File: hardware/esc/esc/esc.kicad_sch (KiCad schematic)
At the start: 9 parts, among them IC1 XMC1100T016F0016ABXUMA1, IC2 STDRIVE101TR, Q1 BSC030P03NS3G, Q2 BSC030P03NS3G, Q3 BSC030P03NS3G, Q4 BSC030P03NS3G, Q5 BSC030P03NS3G, Q6 BSC030P03NS3G, U1 AP62300Z6

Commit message: hardware edits mainly
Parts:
- removed IC1: XMC1100T016F0016ABXUMA1, SOP65P640X120-16N, symbol XMC1100T016F0016ABXUMA1:XMC1100T016F0016ABXUMA1
- removed IC2: STDRIVE101TR, QFN50P400X400X100-25N-D, symbol STDRIVE101TR:STDRIVE101TR
- removed Q1, Q2, Q3, Q4, Q5, Q6: BSC030P03NS3G, BSC0902NSATMA1, symbol BSC030N03LSGATMA1:BSC030P03NS3G
- removed U1: AP62300Z6, Package_TO_SOT_SMD:SOT-563, symbol Regulator_Switching:AP62300Z6
- added C1, C10, C11, C16, C17, C18, C23, C24, C25, C3, C30, C31, C32, C39, C40, C41, C43, C44, C45, C46, C48, C5, C50, C51, C54, C55, C57, C58, C60, C61, C63, C64, C66, C67, C71, C72, C73, C74, C75, C76, C84, C85, C88, C9, C91: 4.7uF, Capacitor_SMD:CP_Elec_6.3x7.7, symbol Device:C_Small
- added C12, C13, C14, C19, C2, C20, C21, C26, C27, C28, C33, C34, C35, C36, C37, C38, C4, C52, C53, C56, C59, C6, C62, C65, C83, C86, C89, C92: 220nF, Capacitor_SMD:C_0402_1005Metric, symbol Device:C_Small
- added C15, C22, C29, C42, C7, C8: 1nF, Capacitor_SMD:C_0603_1608Metric, symbol Device:C_Small
- added C47, C49: 18pF, Capacitor_SMD:C_0402_1005Metric, symbol Device:C_Small
- added C68: 1uF, Capacitor_SMD:C_0603_1608Metric, symbol Device:C_Small
- added C69, C70, C77, C78, C79, C80, C81, C82, C87, C90, C93: 0.1uF, Capacitor_SMD:C_0603_1608Metric, symbol Device:C_Small
- added D1, D10, D11, D12, D13, D14, D15, D16, D17, D18, D19, D2, D3, D4, D5, D6, D7, D8, D9: D_Small, Diode_SMD:D_SMA, symbol Device:D_Small
- added IC1, IC2, IC3, IC4, IC5, IC6: IR2136SPBF, SOIC127P1032X265-28N, symbol IR2136SPBF:IR2136SPBF
- added IC7: TLA2528IRTER, Package_DFN_QFN:WQFN-16-1EP_3x3mm_P0.5mm_EP1.68x1.68mm_ThermalVias, symbol TLA2528IRTER:TLA2528IRTER
- added IC8: MP9486AGN-Z, Package_SO:SOIC-8-1EP_3.9x4.9mm_P1.27mm_EP2.62x3.51mm_ThermalVias, symbol MP9486AGN-Z:MP9486AGN-Z
- added J1: USB-C, Connector_PinHeader_2.54mm:PinHeader_1x04_P2.54mm_Vertical, symbol Connector:Conn_01x04_Pin
- added J10: GPIO, Connector_PinHeader_2.54mm:PinHeader_1x04_P2.54mm_Vertical, symbol Connector:Conn_01x04_Pin
- added J11: Conn_01x08_Pin, Connector_PinHeader_1.27mm:PinHeader_1x08_P1.27mm_Vertical, symbol Connector:Conn_01x08_Pin
- added J2: DEBUG, Connector_PinHeader_2.54mm:PinHeader_1x04_P2.54mm_Vertical, symbol Connector:Conn_01x04_Pin
- added J3: TEMP-GPIO, Connector_PinHeader_1.27mm:PinHeader_1x08_P1.27mm_Vertical, symbol Connector:Conn_01x08_Pin
- added L1: 3.3uH, Inductor_SMD:L_0805_2012Metric_Pad1.05x1.20mm_HandSolder, symbol Device:L_Small
- added L2: 33uH, Inductor_SMD:L_0805_2012Metric, symbol Device:L_Small
- added Q1, Q10, Q11, Q12, Q13, Q14, Q15, Q16, Q17, Q18, Q19, Q2, Q20, Q21, Q22, Q23, Q24, Q25, Q26, Q27, Q28, Q29, Q3, Q30, Q31, Q32, Q33, Q34, Q35, Q36, Q4, Q5, Q6, Q7, Q8, Q9: NMOS, Package_SO:PowerPAK_SO-8L_Single, symbol Simulation_SPICE:NMOS
- added R1, R2, R22, R23, R24, R25, R26, R27, R3, R34, R35, R36, R37, R38, R39, R4, R46, R47, R48, R49, R5, R50, R51, R58, R59, R6, R60, R61, R62, R63, R79, R80, R81, R82, R83, R84: 10, Resistor_SMD:R_1206_3216Metric, symbol Device:R_Small
- added R10, R11, R12, R13, R14, R15, R19, R20, R21, R31, R32, R33, R43, R44, R45, R55, R56, R57, R64, R65, R66, R67, R68, R69, R70, R71, R72, R73, R74, R75, R76, R77, R78: SHUNT, Fuse:Fuse_1206_3216Metric_Pad1.42x1.75mm_HandSolder, symbol Device:R_Small
- added R16, R17, R18, R28, R29, R30, R40, R41, R42, R52, R53, R54, R7, R8, R88, R89, R9, R90: 4.7, Resistor_SMD:R_0805_2012Metric, symbol Device:R_Small
- added R91, R92: 27, Resistor_SMD:R_0402_1005Metric, symbol Device:R_Small
- added R93, R94: 1k, Resistor_SMD:R_0201_0603Metric, symbol Device:R_Small
- added R95: 33, Resistor_SMD:R_1206_3216Metric, symbol Device:R_Small
- added R96: 240k, Resistor_SMD:R_0402_1005Metric, symbol Device:R_Small
- added R97, R98: 10k, Resistor_SMD:R_0402_1005Metric, symbol Device:R_Small
- added SW1, SW2: SW_Push, Connector_PinHeader_2.54mm:PinHeader_1x02_P2.54mm_Vertical, symbol Switch:SW_Push
- added TP1, TP10, TP11, TP12, TP13, TP14, TP15, TP16, TP17, TP18, TP2, TP3, TP4, TP5, TP6, TP7, TP8, TP9: TestPoint_Small, TestPoint:TestPoint_Pad_4.0x4.0mm, symbol Connector:TestPoint_Small
- added TP19, TP20, TP21, TP22: TestPoint, TestPoint:TestPoint_Pad_4.0x4.0mm, symbol Connector:TestPoint
- added U1: RP2354B, Package_DFN_QFN:QFN-80-1EP_10x10mm_P0.4mm_EP3.4x3.4mm, symbol MCU_RaspberryPi:RP2354B
- added U10, U11, U12, U2, U3, U4, U5, U6, U7, U8, U9: INA240A2PW, Package_SO:TSSOP-8_4.4x3mm_P0.65mm, symbol Amplifier_Current:INA240A2PW
- added U14, U15: TMP110D, Package_SON:Texas_X2SON-5_0.8x0.8mm_P0.48mm, symbol Sensor_Temperature:TMP110D
- added U16: AZ1117CH2-3.3, Package_TO_SOT_SMD:SOT-223-3_TabPin2, symbol Regulator_Linear:AZ1117CH2-3.3
- added Y1: 12MHz, Crystal:Crystal_SMD_ECS_CSM3X-2Pin_7.6x4.1mm, symbol Device:Crystal
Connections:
- new net: C49.2, U1.30 (XIN), Y1.2
- new net: C16.1, C19.1, IC3.22 (VS2), Q15.1 (S), Q15.2 (S), Q15.3 (S), Q16.5 (D), TP8.1
- new net: C16.2, C19.2, IC3.24 (VB2), R29.1
- new net: Q10.1 (S), Q10.2 (S), Q10.3 (S), Q12.1 (S), Q12.2 (S), Q12.3 (S), Q8.1 (S), Q8.2 (S), Q8.3 (S), R19.2, R20.2, R21.2, U4.2 (+)
- new net: J1.2 (Pin_2), R91.2
- new net: J1.3 (Pin_3), R92.1
- new net: C11.2, C14.2, IC2.20 (VB3), R18.1
- new net: D5.1 (K), R18.2
- new net: Q4.1 (S), Q4.2 (S), Q4.3 (S), Q5.1 (S), Q5.2 (S), Q5.3 (S), Q6.1 (S), Q6.2 (S), Q6.3 (S), R10.2, R11.2, R12.2, U2.2 (+)
- new net: Q4.4 (G), R4.2
- new net: C5.2, C6.1, IC1.18 (VS3), Q1.1 (S), Q1.2 (S), Q1.3 (S), Q4.5 (D), TP6.1
- new net: C30.1, C33.1, IC5.22 (VS2), Q27.1 (S), Q27.2 (S), Q27.3 (S), Q28.5 (D), TP18.1
- new net: C30.2, C33.2, IC5.24 (VB2), R53.1
- new net: C32.2, C35.2, IC5.20 (VB3), R54.1
- new net: D14.1 (K), R54.2
- new net: C17.1, C20.1, IC3.28 (VB1), R28.1
- new net: C17.2, C20.2, IC3.26 (VS1), Q17.1 (S), Q17.2 (S), Q17.3 (S), Q18.5 (D), TP7.1
- new net: Q35.1 (S), Q35.2 (S), Q35.3 (S), R76.2, R77.2, R78.2, U12.2 (+)
- new net: Q35.4 (G), R84.2
- new net: C36.1, C39.1, IC6.18 (VS3), Q35.5 (D), Q36.1 (S), Q36.2 (S), Q36.3 (S), TP15.1
- new net: IC1.23 (HO2), R2.1
- new net: Q2.4 (G), R2.2
- new net: IC2.15 (LO2), R24.1
- new net: Q10.4 (G), R24.2
- new net: Q28.1 (S), Q28.2 (S), Q28.3 (S), R67.2, R68.2, R69.2, U8.2 (+)
- new net: Q28.4 (G), R60.2
- new net: Q20.1 (S), Q20.2 (S), Q20.3 (S), Q22.1 (S), Q22.2 (S), Q22.3 (S), Q24.1 (S), Q24.2 (S), Q24.3 (S), R43.2, R44.2, R45.2, U6.2 (+)
- new net: C47.2, U1.31 (XOUT), Y1.1
- new net: C29.1, IC5.11 (RCIN)
- new net: R93.2, SW1.1, SW2.1, U1.35 (RUN)
- new net: R94.1, SW2.2
- new net: Q36.4 (G), R83.2
- new net: IC2.23 (HO2), R26.1
- new net: Q9.4 (G), R26.2
- new net: D15.1 (K), R53.2
- new net: C22.1, IC4.11 (RCIN)
- new net: C23.1, C26.1, IC4.22 (VS2), Q21.1 (S), Q21.2 (S), Q21.3 (S), Q22.5 (D), TP11.1
- new net: C23.2, C26.2, IC4.24 (VB2), R41.1
- new net: Q17.4 (G), R39.2
- new net: C31.1, C34.1, IC5.28 (VB1), R52.1
- new net: C31.2, C34.2, IC5.26 (VS1), Q29.1 (S), Q29.2 (S), Q29.3 (S), Q30.5 (D), TP17.1
- new net: C10.2, C13.2, IC2.26 (VS1), Q11.1 (S), Q11.2 (S), Q11.3 (S), Q12.5 (D), TP1.1
- new net: Q31.1 (S), Q31.2 (S), Q31.3 (S), R13.2, R14.2, R15.2, U10.2 (+)
- new net: C25.1, C28.1, IC4.18 (VS3), Q19.1 (S), Q19.2 (S), Q19.3 (S), Q20.5 (D), TP12.1
- new net: Q19.4 (G), R47.2
- new net: IC3.27 (HO1), R39.1
- new net: C12.2, C9.1, IC2.24 (VB2), R17.1
- new net: D6.1 (K), R17.2
- new net: IC5.19 (HO3), R59.1
- new net: Q25.4 (G), R59.2
- new net: Q14.1 (S), Q14.2 (S), Q14.3 (S), Q16.1 (S), Q16.2 (S), Q16.3 (S), Q18.1 (S), Q18.2 (S), Q18.3 (S), R31.2, R32.2, R33.2, U5.2 (+)
- new net: Q18.4 (G), R37.2
- new net: IC7.13 (SCL), U1.12 (GPIO13), U14.2 (SCL), U15.2 (SCL)
- new net: U1.13 (GPIO14), U14.3 (ADD0)
- new net: IC7.14 (SDA), U1.11 (GPIO12), U14.4 (SDA), U15.4 (SDA)
- new net: Q5.4 (G), R5.2
- new net: C3.2, C4.1, IC1.22 (VS2), Q2.1 (S), Q2.2 (S), Q2.3 (S), Q5.5 (D), TP5.1
- new net: C24.2, C27.2, IC4.26 (VS1), Q23.1 (S), Q23.2 (S), Q23.3 (S), Q24.5 (D), TP10.1
- new net: C25.2, C28.2, IC4.20 (VB3), R42.1
- new net: D11.1 (K), R42.2
- new net: C18.1, C21.1, IC3.18 (VS3), Q13.1 (S), Q13.2 (S), Q13.3 (S), Q14.5 (D), TP9.1
- new net: C18.2, C21.2, IC3.20 (VB3), R30.1
- new net: C36.2, C39.2, IC6.20 (VB3), R88.1
- new net: C37.2, C40.2, IC6.26 (VS1), Q31.5 (D), Q32.1 (S), Q32.2 (S), Q32.3 (S), TP13.1
- new net: D9.1 (K), R29.2
- new net: D3.1 (K), R9.2
- new net: Q8.4 (G), R22.2
- new net: C11.1, C14.1, IC2.18 (VS3), Q7.1 (S), Q7.2 (S), Q7.3 (S), Q8.5 (D), TP3.1
- new net: Q33.1 (S), Q33.2 (S), Q33.3 (S), R73.2, R74.2, R75.2, U11.2 (+)
- new net: R55.2, R56.2, R57.2, R64.1, R65.1, R66.1, R67.1, R68.1, R69.1, R70.1, R71.1, R72.1, U7.2 (+)
- new net: Q30.1 (S), Q30.2 (S), Q30.3 (S), R64.2, R65.2, R66.2, U3.2 (+)
- new net: Q6.4 (G), R6.2
- new net: C1.2, C2.2, IC1.26 (VS1), Q3.1 (S), Q3.2 (S), Q3.3 (S), Q6.5 (D), TP4.1
- new net: C1.1, C2.1, IC1.28 (VB1), R8.1
- new net: R93.1, U1.75 (~{QSPI_SS})
- new net: Q29.4 (G), R63.2
- new net: D18.1 (K), R90.2
- new net: C38.1, C41.1, IC6.22 (VS2), Q33.5 (D), Q34.1 (S), Q34.2 (S), Q34.3 (S), TP14.1
- new net: Q34.4 (G), R80.2
- new net: IC8.6 (DIM), IC8.7 (EN), R98.1
- new net: Q26.1 (S), Q26.2 (S), Q26.3 (S), R70.2, R71.2, R72.2, U9.2 (+)
- new net: IC4.23 (HO2), R50.1
- new net: Q21.4 (G), R50.2
- new net: C38.2, C41.2, IC6.24 (VB2), R89.1
- new net: C42.1, IC6.11 (RCIN)
- new net: Q22.4 (G), R48.2
- new net: IC6.15 (LO2), R82.1
- new net: Q33.4 (G), R82.2
- new net: D1.1 (K), R8.2
- new net: D12.1 (K), R41.2
- new net: C44.1, R95.1, U1.61 (VREG_AVDD)
- new net: IC5.14 (LO3), R61.1
- new net: Q30.4 (G), R61.2
- new net: IC4.16 (LO1), R46.1
- new net: Q20.4 (G), R46.2
- new net: Q26.4 (G), R58.2
- new net: C32.1, C35.1, IC5.18 (VS3), Q25.1 (S), Q25.2 (S), Q25.3 (S), Q26.5 (D), TP16.1
- new net: C77.1, U16.2 (GND)
- new net: IC4.15 (LO2), R48.1
- new net: IC7.15 (AIN0/GPIO0), J3.1 (Pin_1)
- new net: IC7.16 (AIN1/GPIO1), J3.2 (Pin_2)
- new net: IC7.1 (AIN2/GPIO2), J3.3 (Pin_3)
- new net: IC7.2 (AIN3/GPIO3), J3.4 (Pin_4)
- new net: IC7.3 (AIN4/GPIO4), J3.5 (Pin_5)
- new net: IC7.4 (AIN5/GPIO5), J3.6 (Pin_6)
- new net: IC7.5 (AIN6/GPIO6), J3.7 (Pin_7)
- new net: IC7.6 (AIN7/GPIO7), J3.8 (Pin_8)
- new net: IC2.14 (LO3), R25.1
- new net: Q12.4 (G), R25.2
- new net: IC1.9 (ITRIP), U1.4 (GPIO7), U2.8
- new net: U1.54 (GPIO43/ADC3), U10.8
- new net: Q31.4 (G), R81.2
- new net: D4.1 (K), R16.2
- new net: C10.1, C13.1, IC2.28 (VB1), R16.1
- new net: IC3.10 (EN), U1.44 (GPIO35)
- new net: C15.1, IC3.11 (RCIN)
- new net: IC3.14 (LO3), R37.1
- new net: IC3.15 (LO2), R36.1
- new net: IC3.16 (LO1), R34.1
- new net: IC3.19 (HO3), R35.1
- new net: IC3.2 (~{HIN1}), IC4.2 (~{HIN1}), IC5.2 (~{HIN1}), U1.38 (GPIO30)
- new net: IC3.23 (HO2), R38.1
- new net: IC3.3 (~{HIN2}), IC4.3 (~{HIN2}), IC5.3 (~{HIN2}), U1.40 (GPIO32)
- new net: IC3.4 (~{HIN3}), IC4.4 (~{HIN3}), IC5.4 (~{HIN3}), U1.43 (GPIO34)
- new net: IC3.5 (~{LIN1}), IC4.5 (~{LIN1}), IC5.5 (~{LIN1}), U1.45 (GPIO36)
- new net: IC3.6 (~{LIN2}), IC4.6 (~{LIN2}), IC5.6 (~{LIN2}), U1.47 (GPIO38)
- new net: IC3.7 (~{LIN3}), IC4.7 (~{LIN3}), IC5.7 (~{LIN3}), U1.48 (GPIO39)
- new net: IC3.8 (~{FAULT}), U1.46 (GPIO37)
- new net: IC3.9 (ITRIP), U1.26 (GPIO25), U5.8
- new net: IC1.14 (LO3), R6.1
- new net: C70.2, IC8.1 (FB), R96.1, R97.2
- new net: Q1.4 (G), R3.2
- new net: C24.1, C27.1, IC4.28 (VB1), R40.1
- new net: Q14.4 (G), R34.2
- new net: C37.1, C40.1, IC6.28 (VB1), R90.1
- new net: D13.1 (K), R52.2
- new net: Q32.4 (G), R79.2
- new net: C68.1, IC7.8 (DECAP)
- new net: IC6.23 (HO2), R80.1
- new net: Q3.4 (G), R1.2
- new net: IC2.10 (EN), U1.9 (GPIO11)
- new net: C8.1, IC2.11 (RCIN)
- new net: IC2.16 (LO1), R22.1
- new net: IC2.19 (HO3), R23.1
- new net: IC1.2 (~{HIN1}), IC2.2 (~{HIN1}), IC6.2 (~{HIN1}), U1.77 (GPIO0)
- new net: C12.1, C9.2, IC2.22 (VS2), Q10.5 (D), Q9.1 (S), Q9.2 (S), Q9.3 (S), TP2.1
- new net: IC2.27 (HO1), R27.1
- new net: IC1.3 (~{HIN2}), IC2.3 (~{HIN2}), IC6.3 (~{HIN2}), U1.79 (GPIO2)
- new net: IC1.4 (~{HIN3}), IC2.4 (~{HIN3}), IC6.4 (~{HIN3}), U1.1 (GPIO4)
- new net: IC1.5 (~{LIN1}), IC2.5 (~{LIN1}), IC6.5 (~{LIN1}), U1.3 (GPIO6)
- new net: IC1.6 (~{LIN2}), IC2.6 (~{LIN2}), IC6.6 (~{LIN2}), U1.6 (GPIO8)
- new net: IC1.7 (~{LIN3}), IC2.7 (~{LIN3}), IC6.7 (~{LIN3}), U1.8 (GPIO10)
- new net: IC2.8 (~{FAULT}), U1.7 (GPIO9)
- new net: IC2.9 (ITRIP), U1.58 (GPIO47/ADC7), U4.8
- new net: D16.1 (K), R89.2
- new net: L1.2, U1.63 (VREG_LX)
- new net: C5.1, C6.2, IC1.20 (VB3), R9.1
- new net: IC4.14 (LO3), R49.1
- new net: Q24.4 (G), R49.2
- new net: IC1.15 (LO2), R5.1
- new net: D17.1 (K), R88.2
- new net: U1.14 (GPIO15), U15.3 (ADD0)
- new net: IC7.11 (ADDR), U1.2 (GPIO5)
- new net: C69.1, D19.1 (K), IC8.5 (SW), L2.2
- new net: C69.2, IC8.4 (BST)
- new net: C3.1, C4.2, IC1.24 (VB2), R7.1
- new net: IC1.19 (HO3), R3.1
- new net: D2.1 (K), R7.2
- new net: IC6.16 (LO1), R84.1
- new net: D10.1 (K), R40.2
- new net: U1.56 (GPIO45/ADC5), U12.8
- new net: Q27.4 (G), R62.2
- new net: IC5.9 (ITRIP), U7.8
- new net: IC6.27 (HO1), R79.1
- new net: IC1.16 (LO1), R4.1
- new net: IC4.27 (HO1), R51.1
- new net: Q23.4 (G), R51.2
- new net: Q16.4 (G), R36.2
- new net: U1.53 (GPIO42/ADC2), U9.8
- new net: Q13.4 (G), R35.2
- new net: IC1.27 (HO1), R1.1
- new net: Q11.4 (G), R27.2
- new net: IC5.27 (HO1), R63.1
- new net: R92.2, U1.67 (USB_DP)
- new net: J11.3 (Pin_3), U1.25 (GPIO24)
- new net: J11.4 (Pin_4), U1.23 (GPIO23)
- new net: J11.5 (Pin_5), U1.22 (GPIO22)
- new net: J11.6 (Pin_6), U1.21 (GPIO21)
- new net: IC4.9 (ITRIP), U1.57 (GPIO46/ADC6), U6.8
- new net: J2.3 (Pin_3), U1.33 (SWCLK)
- new net: J2.4 (Pin_4), U1.34 (SWDIO)
- new net: J10.1 (Pin_1), U1.19 (GPIO19)
- new net: J10.2 (Pin_2), U1.18 (GPIO18)
- new net: J10.3 (Pin_3), U1.17 (GPIO17)
- new net: J10.4 (Pin_4), U1.16 (GPIO16)
- new net: IC4.19 (HO3), R47.1
- new net: IC1.10 (EN), U1.80 (GPIO3)
- new net: C7.1, IC1.11 (RCIN)
- new net: IC1.8 (~{FAULT}), U1.78 (GPIO1)
- new net: IC5.10 (EN), U1.36 (GPIO28)
- new net: IC5.15 (LO2), R60.1
- new net: IC5.16 (LO1), R58.1
- new net: IC5.23 (HO2), R62.1
- new net: IC5.8 (~{FAULT}), U1.37 (GPIO29)
- new net: D7.1 (K), R28.2
- new net: D8.1 (K), R30.2
- new net: Q15.4 (G), R38.2
- new net: R91.1, U1.66 (USB_DM)
- new net: IC4.10 (EN), U1.39 (GPIO31)
- new net: IC4.8 (~{FAULT}), U1.42 (GPIO33)
- new net: IC6.8 (~{FAULT}), U1.27 (GPIO26)
- new net: IC6.10 (EN), U1.28 (GPIO27)
- new net: U1.49 (GPIO40/ADC0), U3.8
- new net: U1.52 (GPIO41/ADC1), U8.8
- new net: U1.55 (GPIO44/ADC4), U11.8
- new net: Q7.4 (G), R23.2
- new net: IC6.14 (LO3), R81.1
- new net: IC6.19 (HO3), R83.1
- new net +1V1: C43.2, C46.2, J2.1 (Pin_1), L1.1, U1.10 (DVDD), U1.32 (DVDD), U1.51 (DVDD), U1.65 (VREG_FB)
- new net +3V3: C45.1, C48.2, C50.1, C51.1, C52.1, C53.1, C54.1, C55.1, C56.1, C57.1, C58.1, C59.1, C60.1, C61.1, C62.1, C63.1, C64.1, C65.1, C66.1, C67.1, C77.2, C78.2, C79.2, C80.2, C81.2, D1.2 (A), D10.2 (A), D11.2 (A), D12.2 (A), D13.2 (A), D14.2 (A), D15.2 (A), D16.2 (A), D17.2 (A), D18.2 (A), D2.2 (A), D3.2 (A), D4.2 (A), D5.2 (A), D6.2 (A), D7.2 (A), D8.2 (A), D9.2 (A), IC1.1 (VCC), IC2.1 (VCC), IC3.1 (VCC), IC4.1 (VCC), IC5.1 (VCC), IC6.1 (VCC), IC7.10 (DVDD), IC7.7 (AVDD), J2.2 (Pin_2), R95.2, U1.15 (IOVDD), U1.24 (IOVDD), U1.29 (IOVDD), U1.41 (IOVDD), U1.5 (IOVDD), U1.50 (IOVDD), U1.59 (ADC_AVDD), U1.60 (IOVDD), U1.64 (VREG_VIN), U1.69 (QSPI_IOVDD), U1.76 (IOVDD), U10.5 (V+), U10.6 (REF2), U11.5 (V+), U11.6 (REF2), U12.5 (V+), U12.6 (REF2), U14.5 (V+), U15.5 (V+), U16.3 (OUT), U2.5 (V+), U2.6 (REF2), U3.5 (V+), U3.6 (REF2), U4.5 (V+), U4.6 (REF2), U5.5 (V+), U5.6 (REF2), U6.5 (V+), U6.6 (REF2), U7.5 (V+), U7.6 (REF2), U8.5 (V+), U8.6 (REF2), U9.5 (V+), U9.6 (REF2)
- new net +5V: C70.1, C71.1, C72.1, C73.1, C74.1, C75.1, C76.1, C82.2, C83.1, C84.1, C85.1, C86.1, C87.2, C88.2, C89.2, C90.1, C91.2, C92.2, C93.1, J1.4 (Pin_4), J11.2 (Pin_2), L2.1, R96.2, U16.1 (IN)
- new net +BATT: IC8.3 (VIN), J11.7 (Pin_7), Q1.5 (D), Q11.5 (D), Q13.5 (D), Q15.5 (D), Q17.5 (D), Q19.5 (D), Q2.5 (D), Q21.5 (D), Q23.5 (D), Q25.5 (D), Q27.5 (D), Q29.5 (D), Q3.5 (D), Q32.5 (D), Q34.5 (D), Q36.5 (D), Q7.5 (D), Q9.5 (D), R98.2, TP20.1, TP21.1
- new net GND: C15.2, C22.2, C29.2, C42.2, C43.1, C44.2, C45.2, C46.1, C47.1, C48.1, C49.1, C50.2, C51.2, C52.2, C53.2, C54.2, C55.2, C56.2, C57.2, C58.2, C59.2, C60.2, C61.2, C62.2, C63.2, C64.2, C65.2, C66.2, C67.2, C68.2, C7.2, C71.2, C72.2, C73.2, C74.2, C75.2, C76.2, C78.1, C79.1, C8.2, C80.1, C81.1, C82.1, C83.2, C84.2, C85.2, C86.2, C87.1, C88.1, C89.1, C90.2, C91.1, C92.1, C93.2, D19.2 (A), IC1.12 (VSS), IC1.13 (COM), IC1.17 (NC_1), IC1.21 (NC_2), IC1.25 (NC_3), IC2.12 (VSS), IC2.13 (COM), IC2.17 (NC_1), IC2.21 (NC_2), IC2.25 (NC_3), IC3.12 (VSS), IC3.13 (COM), IC3.17 (NC_1), IC3.21 (NC_2), IC3.25 (NC_3), IC4.12 (VSS), IC4.13 (COM), IC4.17 (NC_1), IC4.21 (NC_2), IC4.25 (NC_3), IC5.12 (VSS), IC5.13 (COM), IC5.17 (NC_1), IC5.21 (NC_2), IC5.25 (NC_3), IC6.12 (VSS), IC6.13 (COM), IC6.17 (NC_1), IC6.21 (NC_2), IC6.25 (NC_3), IC7.17 (EP), IC7.9 (GND), IC8.8 (GND), IC8.9 (EP), J1.1 (Pin_1), J11.1 (Pin_1), J11.8 (Pin_8), R10.1, R11.1, R12.1, R13.1, R14.1, R15.1, R19.1, R20.1, R21.1, R31.1, R32.1, R33.1, R43.1, R44.1, R45.1, R55.1, R56.1, R57.1, R73.1, R74.1, R75.1, R76.1, R77.1, R78.1, R94.2, R97.1, SW1.2, TP19.1, TP22.1, U1.62 (VREG_PGND), U1.81 (GND), U10.1 (GND), U10.3 (-), U10.4 (GND), U10.7 (REF1), U11.1 (GND), U11.3 (-), U11.4 (GND), U11.7 (REF1), U12.1 (GND), U12.3 (-), U12.4 (GND), U12.7 (REF1), U14.1 (GND), U15.1 (GND), U2.1 (GND), U2.3 (-), U2.4 (GND), U2.7 (REF1), U3.1 (GND), U3.3 (-), U3.4 (GND), U3.7 (REF1), U4.1 (GND), U4.3 (-), U4.4 (GND), U4.7 (REF1), U5.1 (GND), U5.3 (-), U5.4 (GND), U5.7 (REF1), U6.1 (GND), U6.3 (-), U6.4 (GND), U6.7 (REF1), U7.1 (GND), U7.3 (-), U7.4 (GND), U7.7 (REF1), U8.1 (GND), U8.3 (-), U8.4 (GND), U8.7 (REF1), U9.1 (GND), U9.3 (-), U9.4 (GND), U9.7 (REF1)

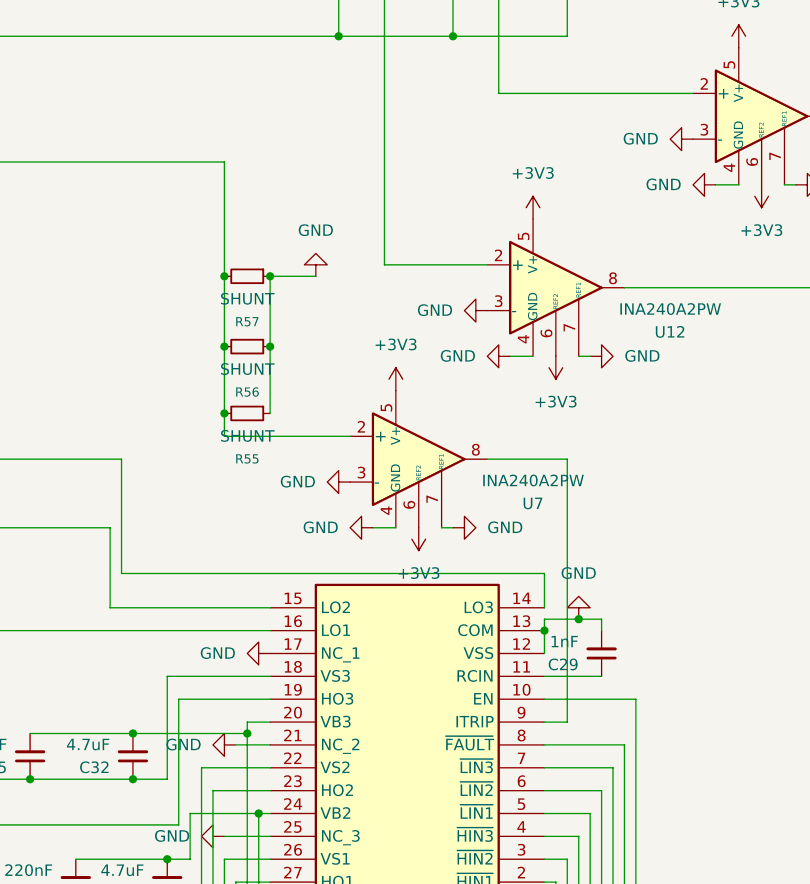
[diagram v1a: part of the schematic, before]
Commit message: block 1x1
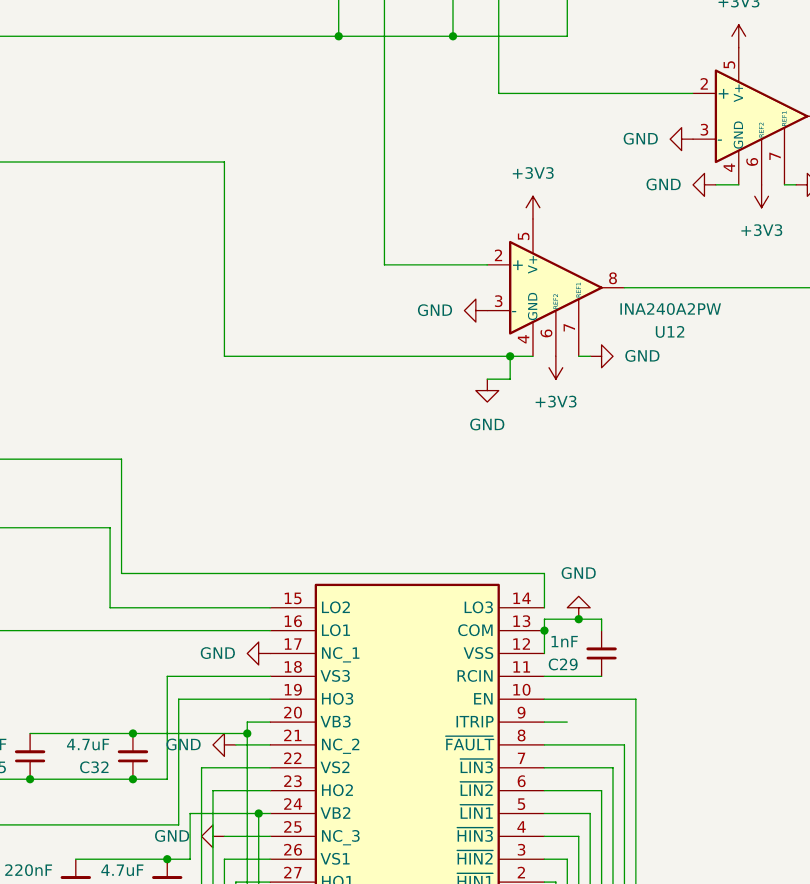
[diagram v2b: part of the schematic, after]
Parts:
- removed R55, R56, R57: SHUNT, Fuse:Fuse_1206_3216Metric_Pad1.42x1.75mm_HandSolder, symbol Device:R_Small
- removed U7: INA240A2PW, Package_SO:TSSOP-8_4.4x3mm_P0.65mm, symbol Amplifier_Current:INA240A2PW
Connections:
- net GND: now also R64.1, R65.1, R66.1, R67.1, R68.1, R69.1, R70.1, R71.1, R72.1
